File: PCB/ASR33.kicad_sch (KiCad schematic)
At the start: 44 parts, among them J1 Shelly, J2 DC, J3 Power, J4 RUN, J5 Tx, J6 Rx, J7 USB-C, Q1 NX7002AK, SW1 SW_Push, U1 ESP32-PICO-MINI-02, U2 FT231XQ, U3 NCR402U, U4 NCR402U, U5 LTV-356T, U6 LMR16006XDDCR, U7 QR

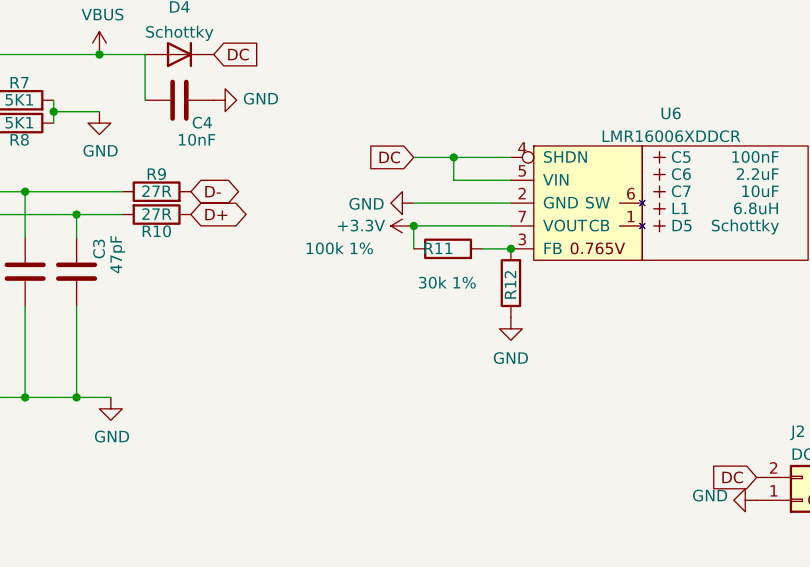
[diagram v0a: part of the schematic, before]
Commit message: Tidy silk
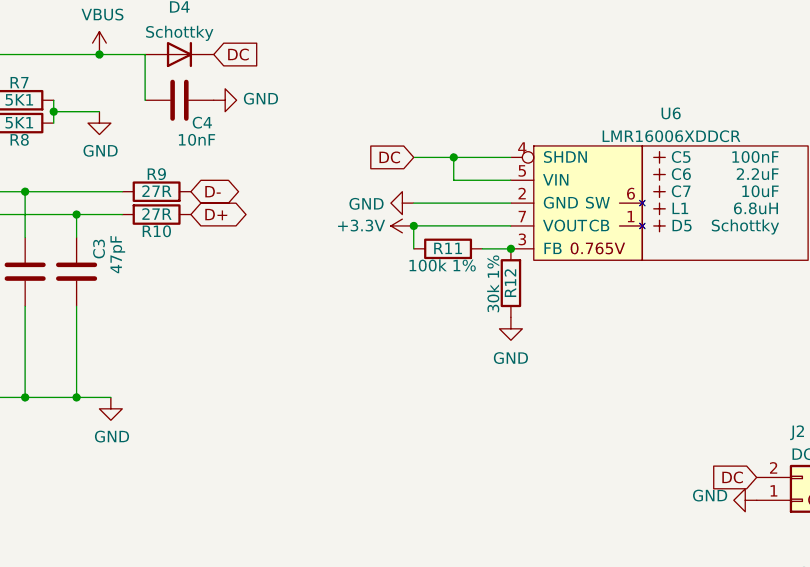
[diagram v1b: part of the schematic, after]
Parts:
- D5: JLCPCB Rotation Offset 0 -> (none)
- Q1: footprint Package_TO_SOT_SMD:SOT-23 -> RevK:SOT-23
- U5: footprint Package_SO:SO-4_4.4x3.6mm_P2.54mm -> RevK:SO-4_4.4x3.6mm_P2.54mm
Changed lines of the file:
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@@
   (symbol (lib_id "Device:R") (at 231.775 50.8 180) (unit 1)
     (in_bom yes) (on_board yes) (dnp no)
-    (property "Reference" "R12" (at 231.775 52.705 90)
-      (effects (font (size 1.27 1.27)) (justify right))
-    )
-    (property "Value" "30k 1%" (at 227.965 50.8 0)
+    (property "Reference" "R12" (at 231.775 50.8 90)
+      (effects (font (size 1.27 1.27)))
+    )
+    (property "Value" "30k 1%" (at 229.87 47.625 90)
       (effects (font (size 1.27 1.27)) (justify left))
     )
@@
       (effects (font (size 1.27 1.27)))
     )
-    (property "Footprint" "Package_SO:SO-4_4.4x3.6mm_P2.54mm" (at 234.95 144.78 0)
+    (property "Footprint" "RevK:SO-4_4.4x3.6mm_P2.54mm" (at 234.95 144.78 0)
       (effects (font (size 1.27 1.27) italic) (justify left) hide)
     )
@@
       (effects (font (size 1.27 1.27)) (justify left))
     )
-    (property "Footprint" "Package_TO_SOT_SMD:SOT-23" (at 231.775 113.665 0)
+    (property "Footprint" "RevK:SOT-23" (at 231.775 113.665 0)
       (effects (font (size 1.27 1.27)) hide)
     )
@@
   (symbol (lib_id "Device:R") (at 224.79 46.99 90) (unit 1)
     (in_bom yes) (on_board yes) (dnp no)
-    (property "Reference" "R11" (at 225.425 46.99 90)
-      (effects (font (size 1.27 1.27)) (justify left))
-    )
-    (property "Value" "100k 1%" (at 216.535 46.99 90)
+    (property "Reference" "R11" (at 224.79 46.99 90)
+      (effects (font (size 1.27 1.27)))
+    )
+    (property "Value" "100k 1%" (at 227.965 48.895 90)
       (effects (font (size 1.27 1.27)) (justify left))
     )
@@
       (effects (font (size 1.27 1.27)) hide)
     )
-    (property "JLCPCB Rotation Offset" "0" (at 248.285 44.45 0)
-      (effects (font (size 1.27 1.27)) hide)
-    )
